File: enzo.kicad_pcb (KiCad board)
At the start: 2 copper layers, 118 x 95.1 mm, 63 parts, among them SW1 SW_Push, SW10 SW_Push, SW11 SW_Push, SW12 SW_Push, SW13 SW_Push, SW14 SW_Push, SW15 SW_Push, SW16 SW_Push, SW17 locked, SW2 SW_Push, SW3 SW_Push, SW4 SW_Push, SW5 SW_Push, SW6 SW_Push, SW7 SW_Push, SW8 SW_Push, SW9 SW_Push

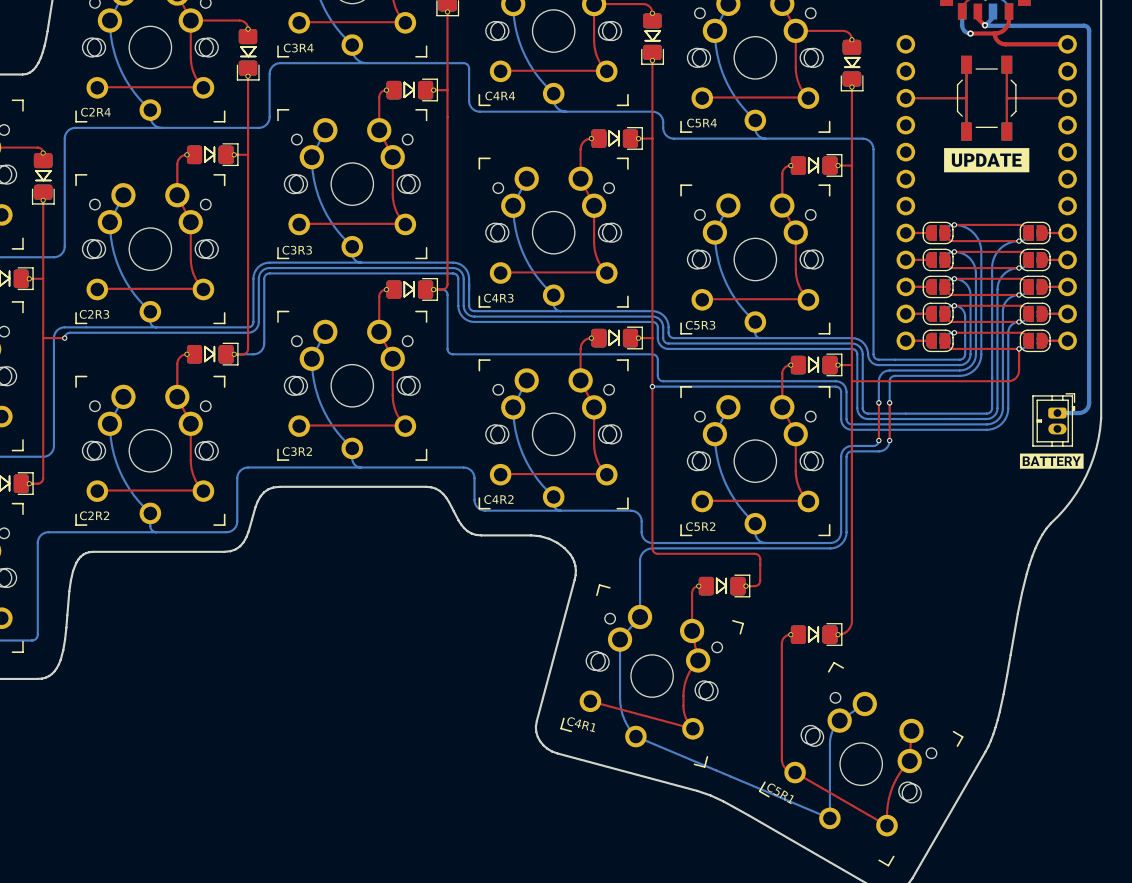
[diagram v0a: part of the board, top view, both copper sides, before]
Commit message: Minor trace tweaks/cleanup
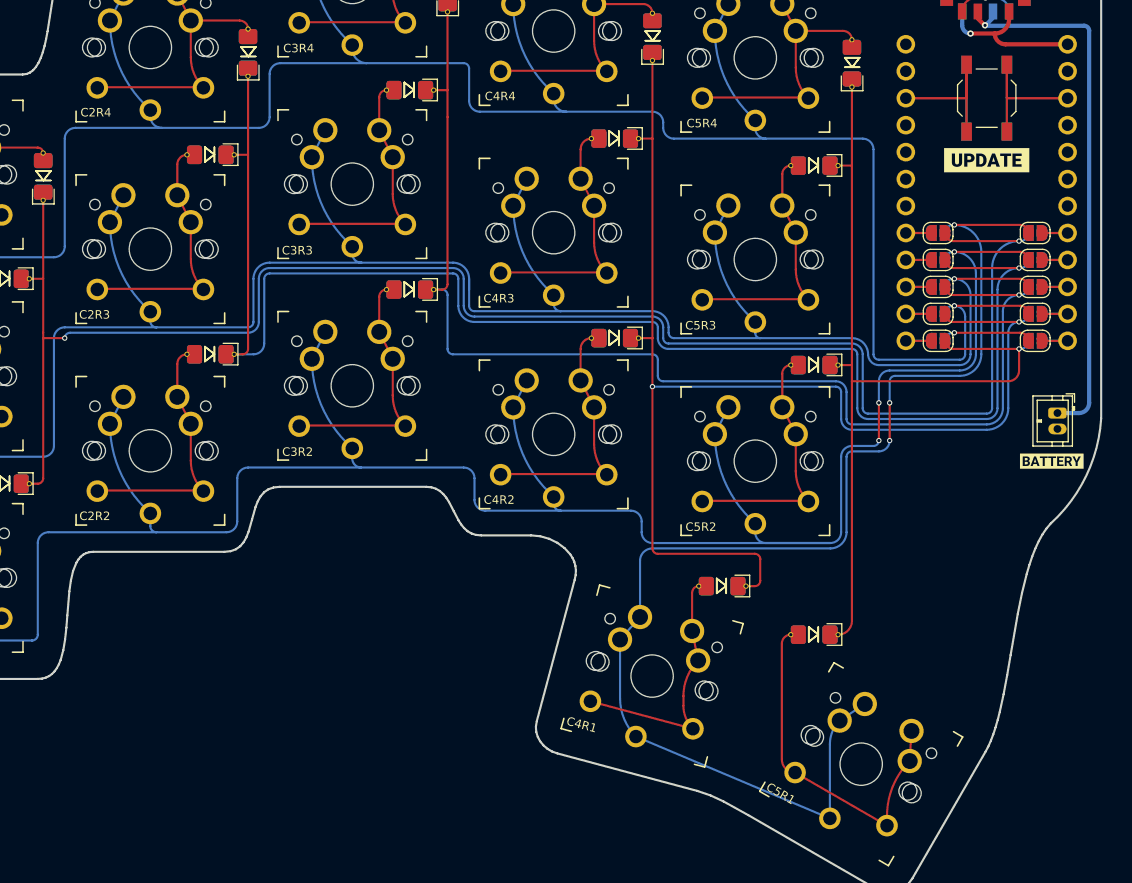
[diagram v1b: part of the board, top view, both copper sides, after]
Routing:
- net grnd: track 24.2 -> 30.3 mm
- net rst: track 24.2 -> 30.3 mm
- net row2_matrix: track 226.8 -> 232.4 mm
- net col2_matrix: track 148.0 -> 147.0 mm
- net col1_matrix: track 166.6 -> 166.1 mm
- net row3_matrix: track 211.6 -> 212.1 mm
